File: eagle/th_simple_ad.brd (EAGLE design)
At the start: 100 x 80 mm, 24 parts, among them IC1 TL071P, IC2 LM555N, T1 2N3904

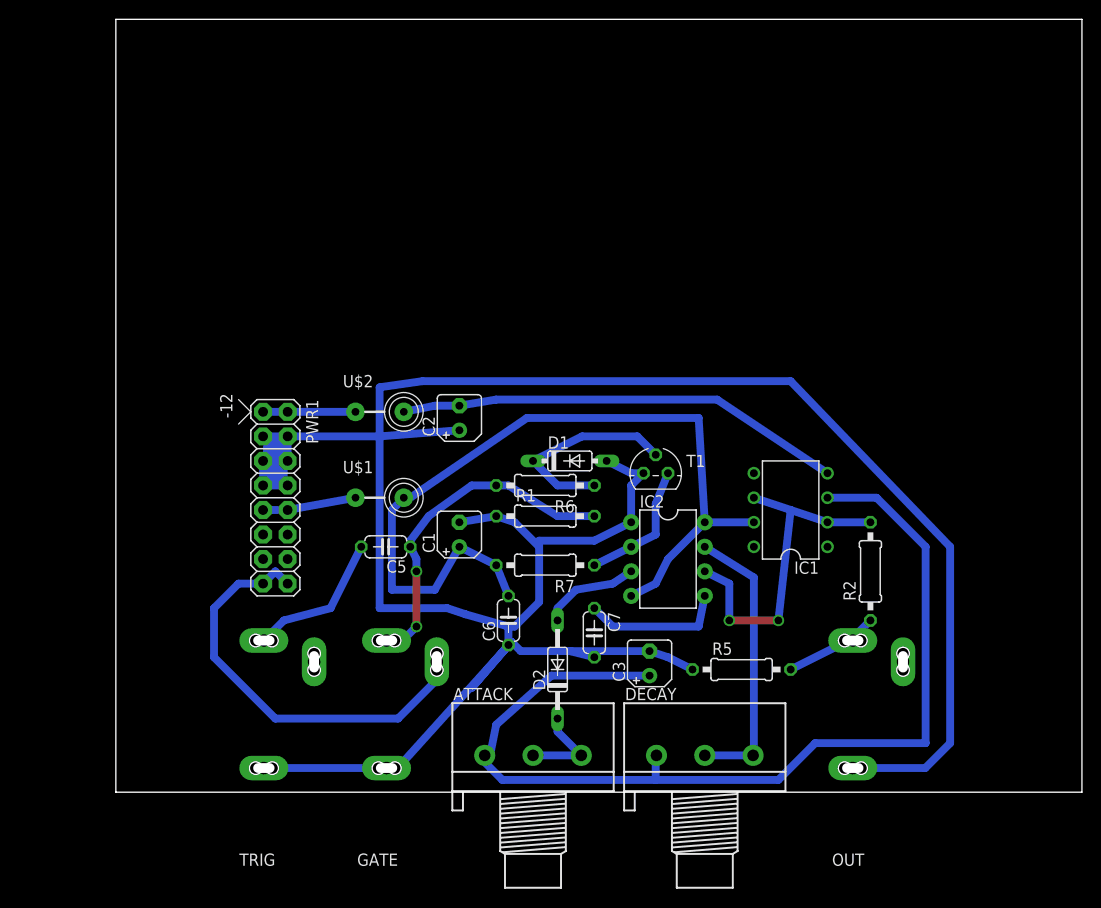
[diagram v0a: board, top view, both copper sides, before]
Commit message: vertical and cutout
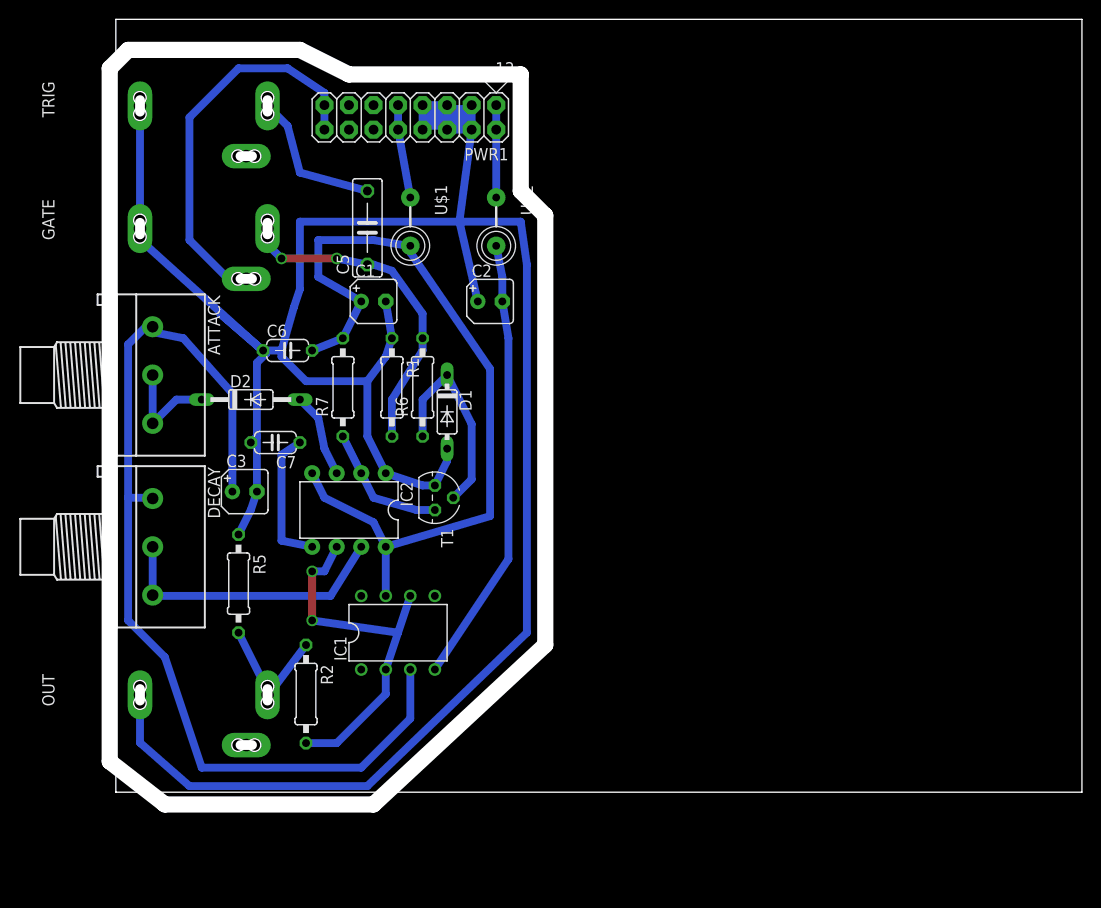
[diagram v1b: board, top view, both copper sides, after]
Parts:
- C5: device rcl:C050-024X044 -> rcl:C075-032X103
- moved OUT 81.4 mm to (0.00, 5.08), turned to 90 degrees
- moved TRIG 69.1 mm to (0.00, 66.0), turned to 90 degrees
- moved GATE 62.7 mm to (0.00, 53.3), turned to 90 degrees
- moved DECAY 61.1 mm to (3.81, 25.4), turned to 270 degrees
- moved R2 59.8 mm to (19.7, 10.2), turned to 270 degrees
- moved ATTACK 55.7 mm to (3.81, 43.2), turned to 270 degrees
- moved R5 52.8 mm to (12.7, 21.6), turned to 270 degrees
- moved C3 45.5 mm to (13.3, 31.1), turned to 0 degrees
- moved IC1 42.6 mm to (29.2, 16.5), turned to 0 degrees
- moved D2 42.3 mm to (14.0, 40.6), turned to 0 degrees
- moved PWR1 40.4 mm to (33.0, 69.8), turned to 180 degrees
- moved C7 38.4 mm to (16.5, 36.2), turned to 180 degrees
- moved C6 36.1 mm to (17.8, 45.7), turned to 0 degrees
- moved IC2 33.4 mm to (24.1, 29.2), turned to 180 degrees
- moved C5 33.1 mm to (26.0, 58.4), turned to 90 degrees
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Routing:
- net GND: track 272.2 -> 267.9 mm
- net N$3: track 10.0 -> 13.7 mm
- net N$5: track 35.7 -> 39.1 mm
- net N$16: track 105.8 -> 102.6 mm
- net N$12: track 44.0 -> 40.9 mm
- net +12V: track 87.4 -> 84.5 mm
- net N$8: track 10.1 -> 8.77 mm
- net N$9: track 9.83 -> 11.1 mm
- net N$14: track 35.0 -> 34.4 mm
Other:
- board size 100 x 80 mm -> 100.6 x 81.3 mm

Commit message: verified
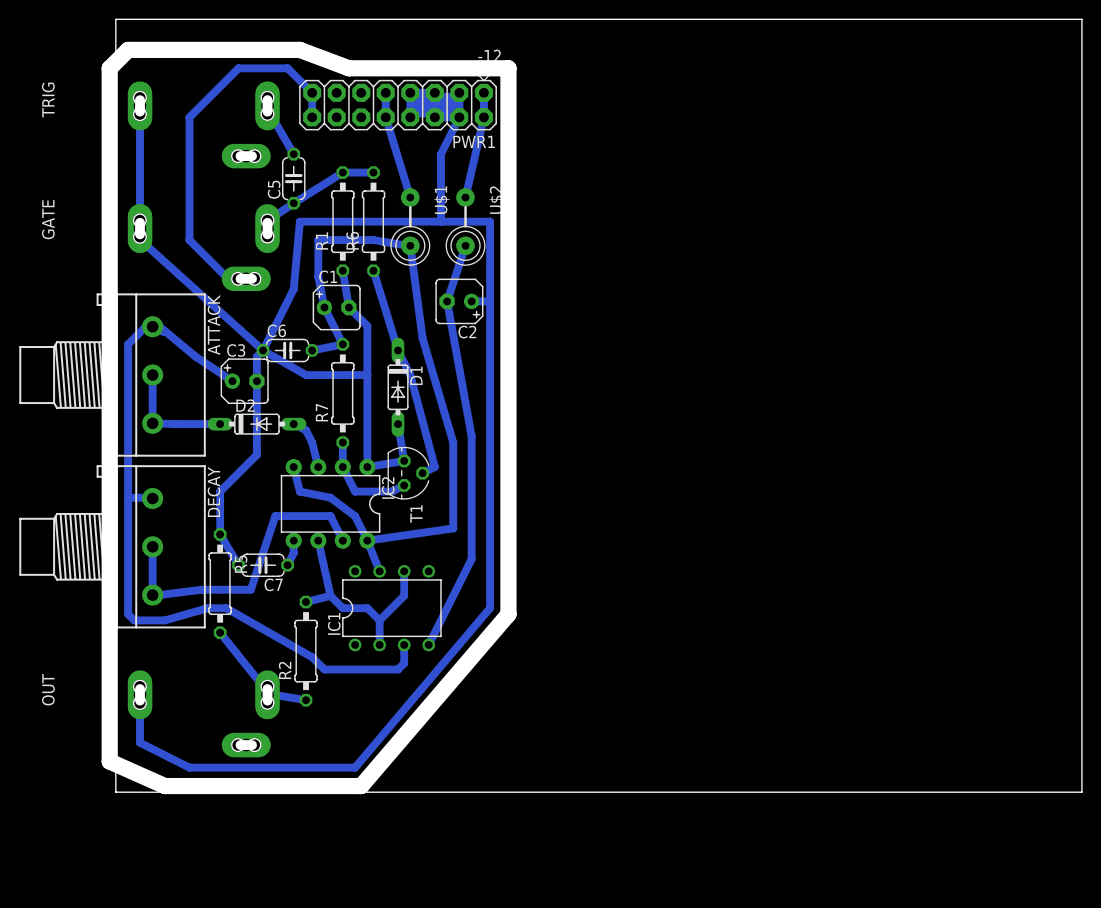
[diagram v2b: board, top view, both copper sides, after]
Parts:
- C5: device rcl:C075-032X103 -> rcl:C050-024X044
- D2: value 1N4148DO35-10 -> 1N4148DO35-7; device diode:DO35-10 -> diode:DO35-7
- moved R1 17.9 mm to (23.5, 59.1), turned to 90 degrees
- moved R6 17.9 mm to (26.7, 59.1)
- moved C7 12.8 mm to (15.2, 23.5)
- moved C3 11.4 mm to (13.3, 42.5)
- moved C5 9.16 mm to (18.4, 63.5)
- moved D1 5.68 mm to (29.2, 41.9)
- moved R2 4.45 mm to (19.7, 14.6), turned to 90 degrees
- moved T1 4.07 mm to (29.8, 33.0)
- moved C1 3.86 mm to (22.9, 50.2)
- moved C2 3.17 mm to (35.6, 50.8), turned to 180 degrees
- moved U$2 3.17 mm to (36.2, 59.1)
- moved IC1 2.62 mm to (28.6, 19.1)
- moved D2 2.62 mm to (14.6, 38.1)
- moved IC2 2.01 mm to (22.2, 29.8)
- moved R5 1.90 mm to (10.8, 21.6)
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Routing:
- net GND: track 267.9 -> 245.1 mm
- net N$16: track 102.6 -> 80.1 mm
- net N$14: track 34.4 -> 13.6 mm, vias 2 -> 0
- net N$5: track 39.1 -> 23.3 mm, vias 2 -> 0
- net N$10: track 14.4 -> 2.69 mm
- net N$13: track 15.2 -> 6.97 mm
- net +12V: track 84.5 -> 78.2 mm
- net -12V: track 46.3 -> 42.9 mm
- net N$8: track 8.77 -> 5.46 mm
- net N$7: track 13.6 -> 10.6 mm
- net N$11: track 29.5 -> 31.9 mm
- net N$12: track 40.9 -> 38.6 mm
- net N$1: track 9.68 -> 11.2 mm
- net N$2: track 9.57 -> 11.1 mm
- net N$3: track 13.7 -> 12.2 mm
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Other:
- board size 100.6 x 81.3 mm -> 100.6 x 80 mm
